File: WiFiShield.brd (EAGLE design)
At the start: 69.2 x 53.3 mm, 39 parts, among them IC1 MIC5219-3.3YM5, IC2 CC3000, J7 Arduino-compatible headers, Q1 2N7002, Q2 2N7002, Q3 2N7002, Q4 2N7002, Q5 2N7002

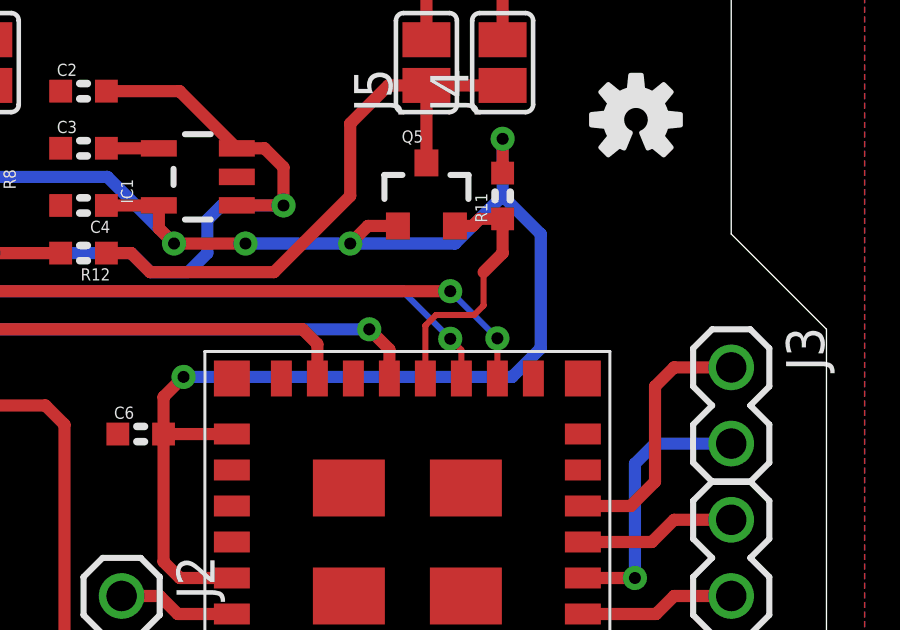
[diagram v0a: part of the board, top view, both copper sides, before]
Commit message: foo
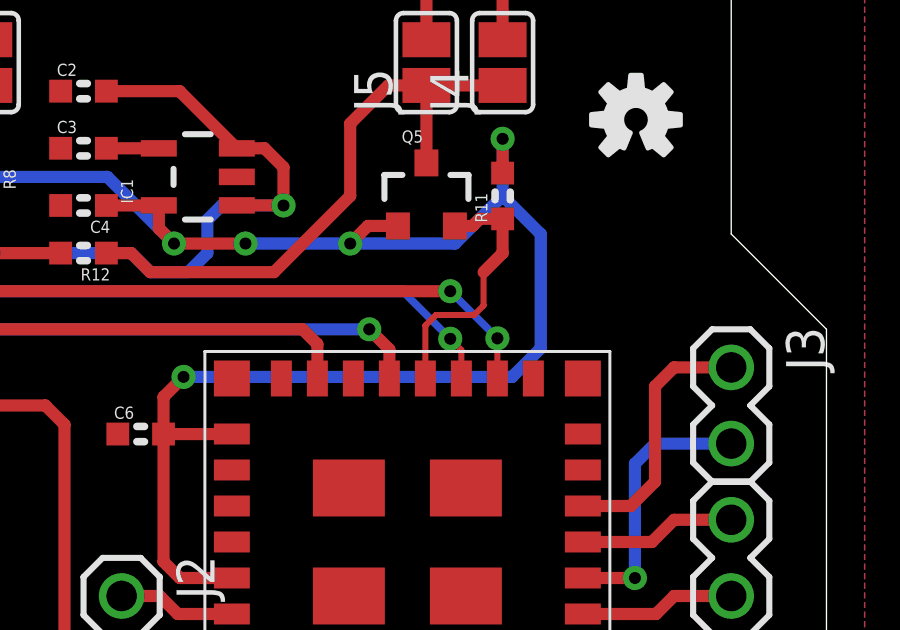
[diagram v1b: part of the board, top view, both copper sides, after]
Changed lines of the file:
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@@
 <via x="33.02" y="39.37" extent="1-16" drill="0.4"/>
 <wire x1="33.02" y1="39.37" x2="55.08625" y2="39.37" width="0.4064" layer="16"/>
-<wire x1="55.08625" y1="39.37" x2="56.67375" y2="37.7825" width="0.2032" layer="16"/>
+<wire x1="55.08625" y1="39.37" x2="56.67375" y2="37.7825" width="0.254" layer="16"/>
 <wire x1="57.045" y1="36.46" x2="57.045" y2="37.41125" width="0.2032" layer="1"/>
 <wire x1="57.045" y1="37.41125" x2="56.67375" y2="37.7825" width="0.2032" layer="1"/>
@@
 <wire x1="39.6875" y1="41.5425" x2="39.685" y2="41.545" width="0.4064" layer="1"/>
 <wire x1="39.497" y1="39.37" x2="56.67375" y2="39.37" width="0.4064" layer="1"/>
-<wire x1="56.67375" y1="39.37" x2="58.245" y2="37.79875" width="0.2032" layer="16"/>
+<wire x1="56.67375" y1="39.37" x2="58.245" y2="37.79875" width="0.254" layer="16"/>
 <wire x1="58.245" y1="36.46" x2="58.245" y2="37.79875" width="0.2032" layer="1"/>
 <via x="56.67375" y="39.37" extent="1-16" drill="0.4"/>
